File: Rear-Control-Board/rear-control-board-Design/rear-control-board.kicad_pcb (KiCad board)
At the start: 2 copper layers, 139 x 104.8 mm, 59 parts, among them J1 Conn_01x23, J2 Conn_01x23, J3 Conn_01x08, J4 JST-B2B-VERT-2PIN, J5 JST-B2B-VERT-2PIN, J6 Conn_01x02, J7 Micro_SD_Card, K1 T9VV1K15-12S, K2 G5V-2, K3 G5V-2, K4 G5V-1, K5 G5V-1, K6 G5V-1, Q1 2N7002, U1 Dev_Board_C, U2 TS2940CP33_ROG, U4 MAX33054EASA+T

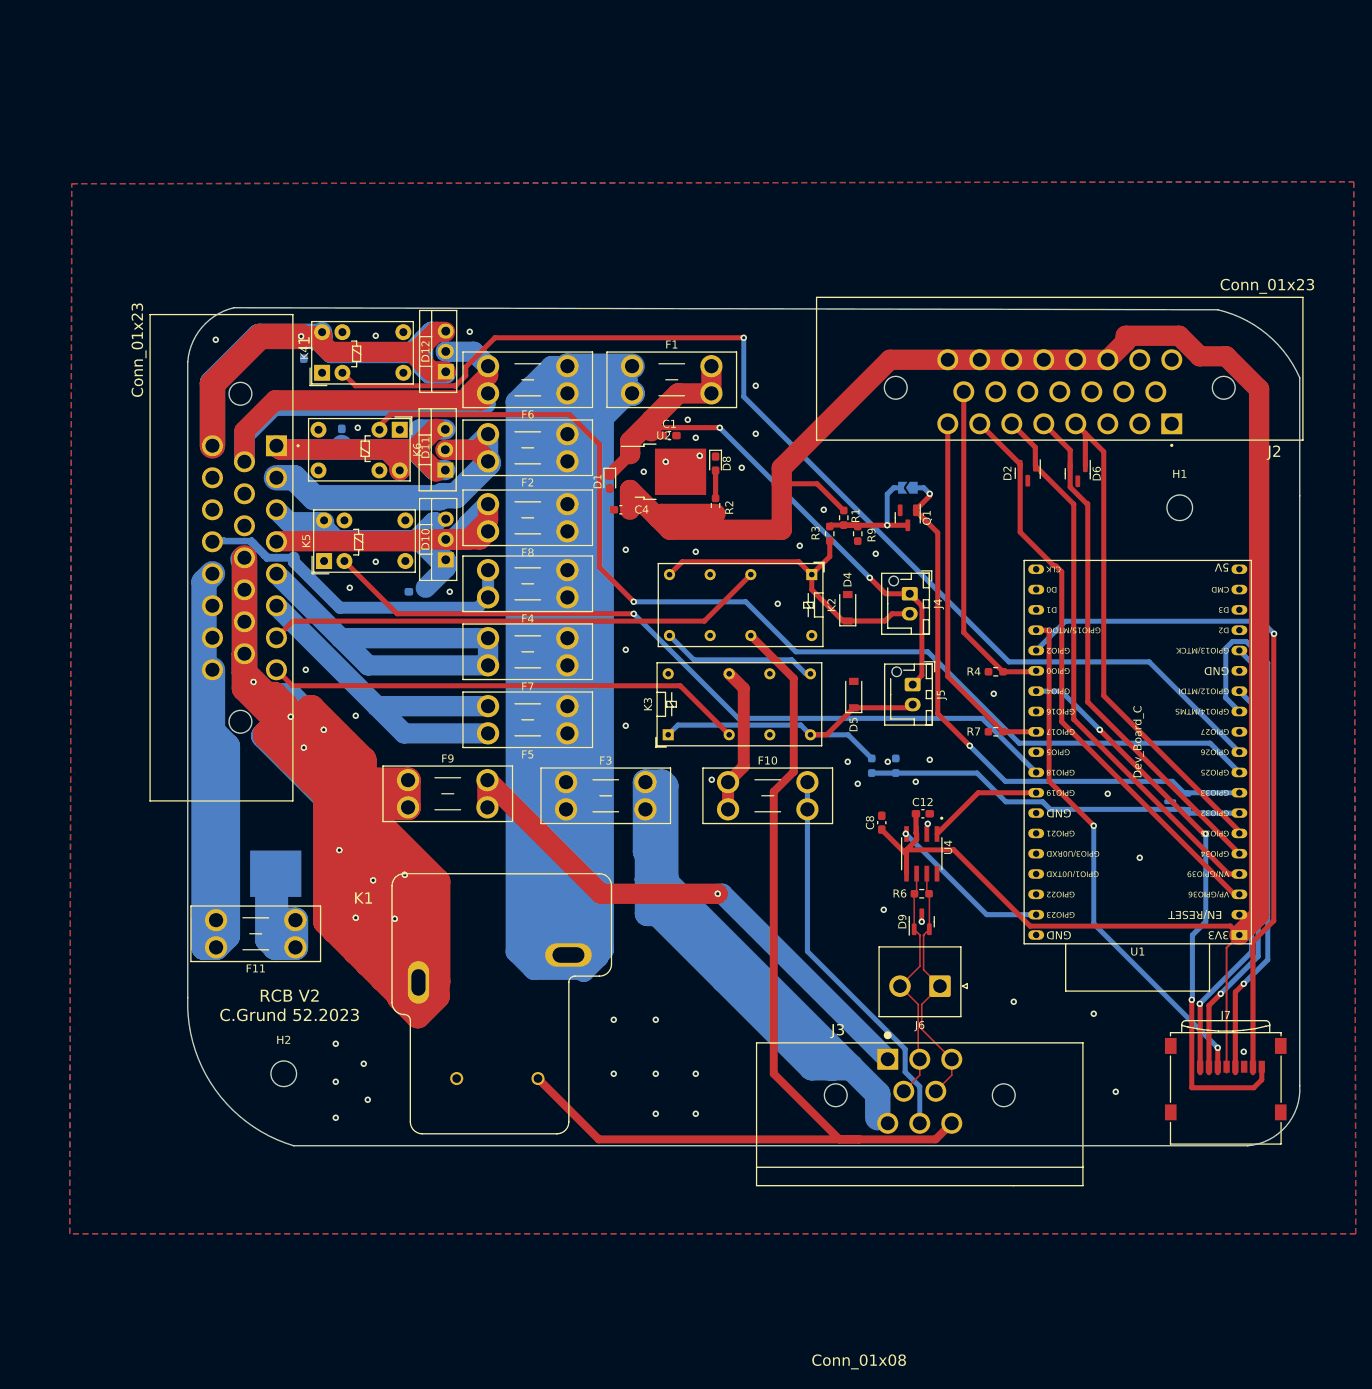
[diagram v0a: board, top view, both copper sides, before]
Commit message: OOPSIE
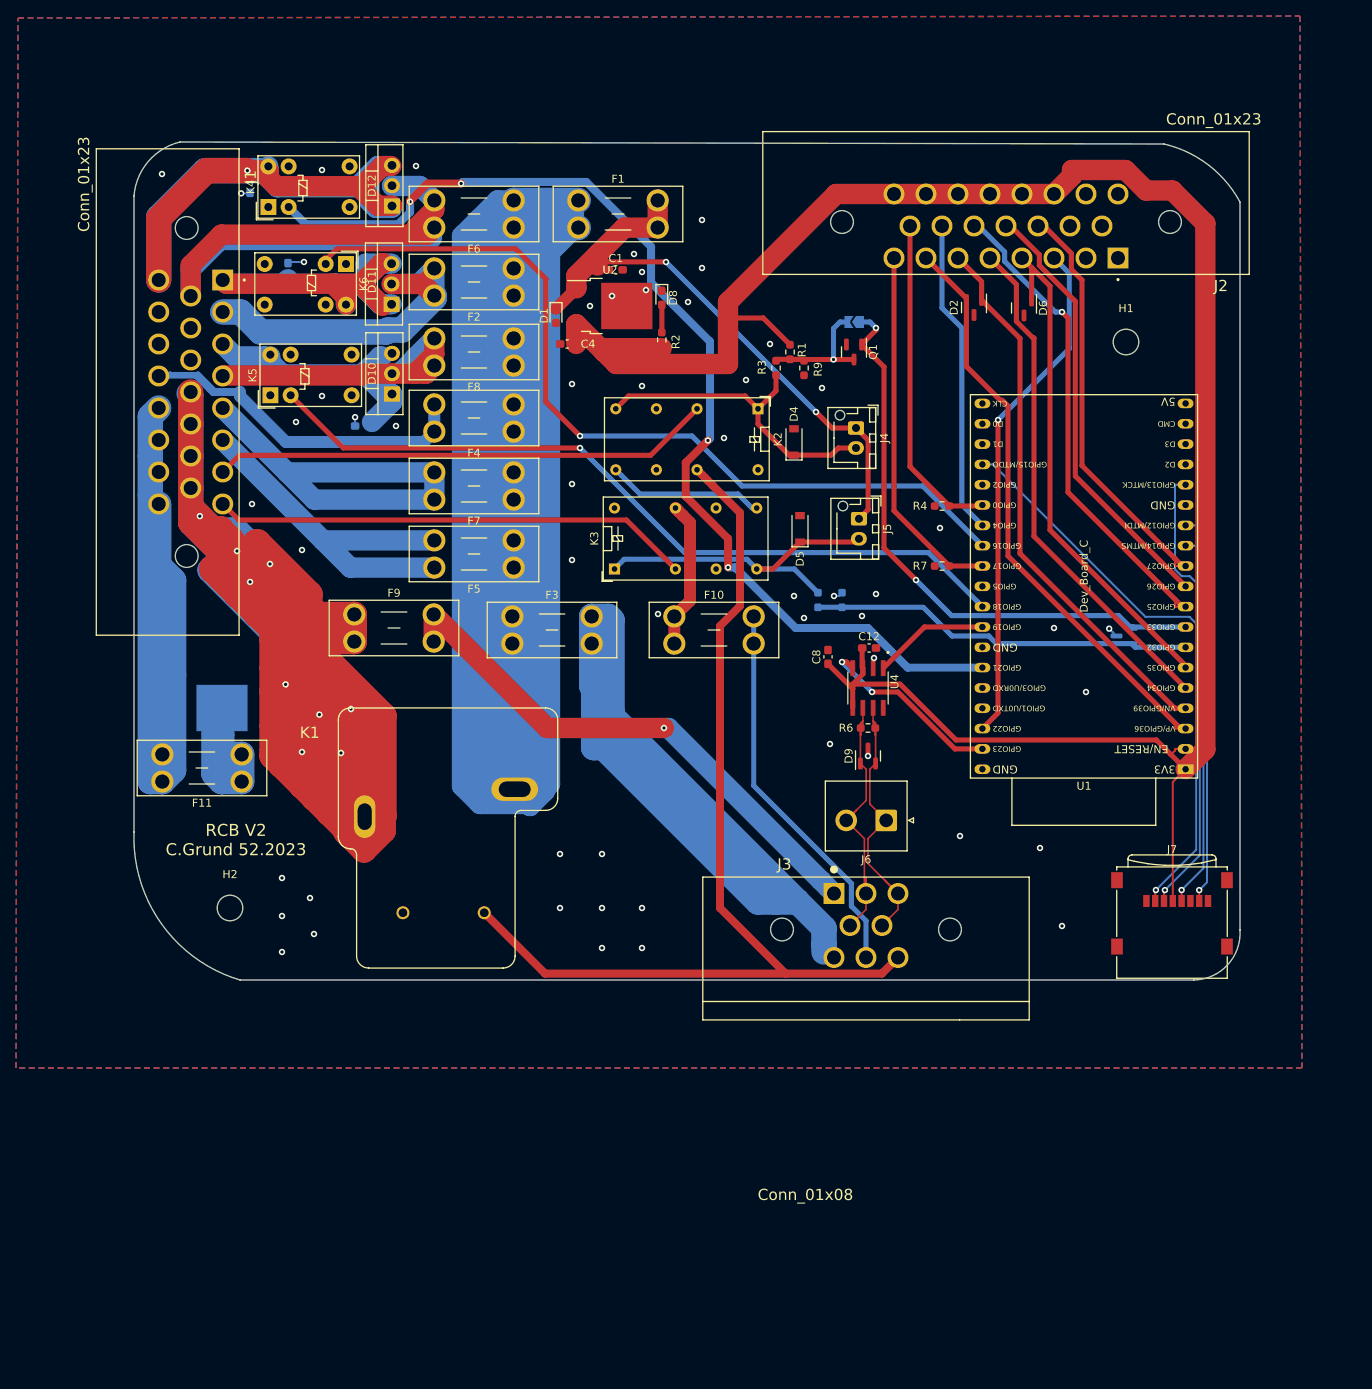
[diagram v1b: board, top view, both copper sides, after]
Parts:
- moved U1 21.8 mm to (183.2, 117.7)
- moved D5 21.8 mm to (135.0, 87.6)
- moved J5 21.8 mm to (142.4, 86.4)
- moved K2 21.8 mm to (129.8, 72.6)
- moved K3 21.8 mm to (111.8, 92.7)
- moved J6 21.8 mm to (145.8, 124.1)
- moved F10 21.8 mm to (119.3, 98.6)
- moved F3 21.8 mm to (99.1, 98.6)
- moved F9 21.8 mm to (79.3, 98.3)
- moved C12 21.8 mm to (143.7, 102.5)
- moved C3 21.8 mm to (80.3, 74.8)
- moved C4 21.8 mm to (105.9, 64.5)
- moved C8 21.8 mm to (138.5, 103.6)
- moved D10 21.8 mm to (84.0, 70.8)
- moved D11 21.8 mm to (84.0, 59.6)
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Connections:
- net /Controller/CLK renamed /Controller/SD_CLK
- J2 pad 11: unconnected-(J2-Pad11) -> PAC1_1
- J2 pad 12: unconnected-(J2-Pad12) -> PAC1_2
- J2 pad 13: unconnected-(J2-Pad13) -> PAC2_1
- J2 pad 14: unconnected-(J2-Pad14) -> PAC2_2
- J2 pad 3: unconnected-(J2-Pad3) -> BMS_Therm_Out
- J7 pad 1: /Controller/DAT2 -> unconnected-(J7-Pad1)
- J7 pad 2: /Controller/DAT3 -> /Controller/CS_SD
- J7 pad 3: /Controller/CMD -> /Controller/SD_MOSI
- J7 pad 7: /Controller/DAT0 -> /Controller/SD_MISO
- J7 pad 8: /Controller/DAT1 -> unconnected-(J7-Pad8)
- U1 pad 10: /Controller/FAN_CTRL -> PAC1_2
- U1 pad 11: unconnected-(U1-Pad11) -> PAC1_1
- U1 pad 13: /Controller/DAT2 -> /Controller/SD_MISO
- U1 pad 15: /Controller/DAT3 -> /Controller/SD_MOSI
- U1 pad 23: /Controller/CMD -> /Controller/CS_SD
- U1 pad 24: /Controller/DAT0 -> unconnected-(U1-Pad24)
- U1 pad 26: /Controller/DAT1 -> PAC2_2
- U1 pad 27: unconnected-(U1-Pad27) -> /Controller/BRAKE_CTRL
- U1 pad 33: unconnected-(U1-Pad33) -> /Controller/FAN_CTRL
- U1 pad 36: unconnected-(U1-Pad36) -> BMS_Therm_Out
- U1 pad 9: /Controller/BRAKE_CTRL -> PAC2_1
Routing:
- net /Controller/DAT0: track 87.9 -> 0.00 mm, vias 1 -> 0
- net /Controller/DAT1: track 71.9 -> 0.00 mm, vias 3 -> 0
- net /Controller/CS_SD: track 0.00 -> 71.8 mm, vias 0 -> 1
- net /Controller/CMD: track 65.6 -> 0.00 mm, vias 2 -> 0
- net BMS_Therm_Out: track 0.00 -> 64.1 mm, vias 0 -> 1
- net PAC2_1: track 0.00 -> 61.5 mm, vias 0 -> 1
- net /Controller/SD_MOSI: track 0.00 -> 57.1 mm, vias 0 -> 1
- net /Controller/DAT3: track 56.3 -> 0.00 mm, vias 1 -> 0
- net PAC1_2: track 0.00 -> 54.7 mm
- net PAC1_1: track 0.00 -> 52.7 mm
- net /Controller/DAT2: track 51.0 -> 0.00 mm, vias 1 -> 0
- net /Controller/SD_MISO: track 0.00 -> 49.2 mm, vias 0 -> 1
- net PAC2_2: track 0.00 -> 39.5 mm
- net /Controller/BRAKE_CTRL: track 136.1 -> 107.5 mm
- net /Controller/SD_CLK: track 68.2 -> 47.2 mm
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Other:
- board size 139 x 104.8 mm -> 138.3 x 104.8 mm
